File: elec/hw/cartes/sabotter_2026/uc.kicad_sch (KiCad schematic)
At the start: 34 parts, among them J3 USB4105-GF-A-060, SW1 TSB001A3526A02, U3 ESP32-S3-WROOM-1

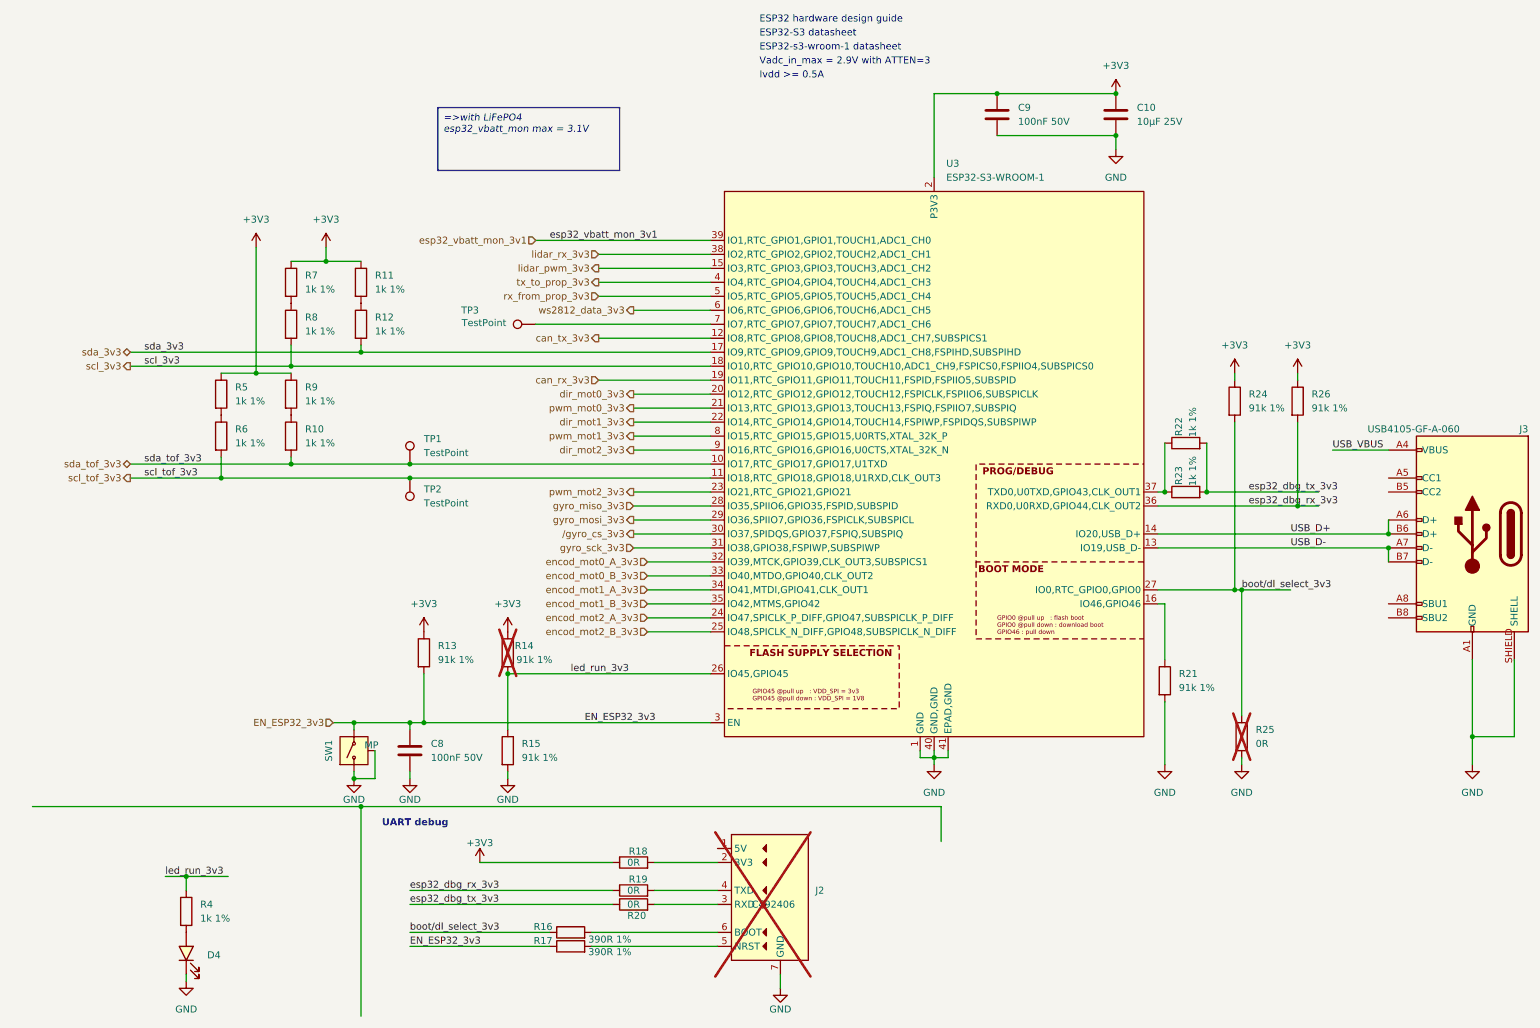
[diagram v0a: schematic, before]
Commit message: sabotter wip
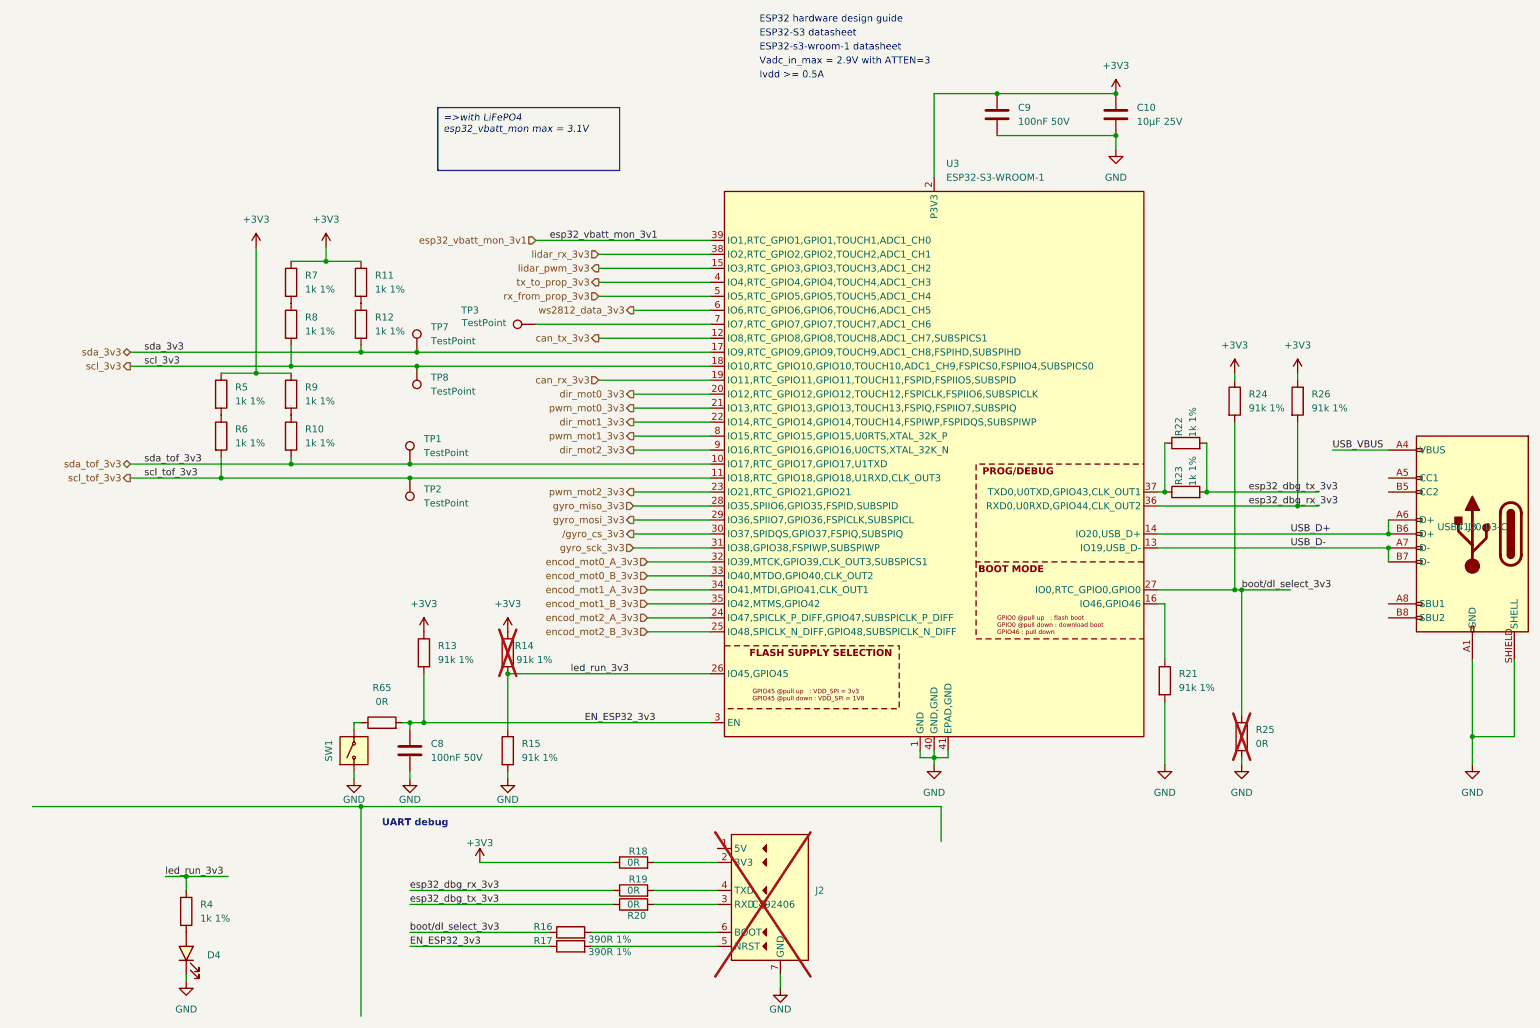
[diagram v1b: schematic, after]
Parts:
- added R65: 0R, cocotter_resistor:r0603_reflow, symbol cocotter_resistors:R_0R_0603
- added TP7, TP8: TestPoint, cocotter_others:testpoint-THT-0.5mm, symbol cocotter_others:TestPoint
- J3: value USB4105-GF-A-060 -> USB4120-03-C; footprint cocotter_connectors:USB4105 -> cocotter_connectors:USB4120-03-C; symbol cocotter_connectors:USB-TYPE-C-019 -> cocotter_connectors:USB4120-03-C; DIGIKEY_REF 2073-USB4105-GF-A-060TR-ND -> (none); JLC (none) -> C7450621; JLCPCB Part # C2927039 -> (none)
- SW1: value TSB001A3526A02 -> PTS525 SK15 SMTR2 LFS; footprint cocotter_others:TSB001A3526A02 -> cocotter_others:PTS525 SK15 SMTR2 LFS; symbol cocotter_others:TSB001A3526A02 -> cocotter_others:PTS525 SK15 SMTR2 LFS; JLCPCB Part # C2888889 -> C2689599
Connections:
- net EN_ESP32_3v3: now also R65.2; no longer SW1.2
- net GND: now also SW1.A (1); no longer SW1.1, SW1.MP
- net scl_3v3: now also TP8.1
- net sda_3v3: now also TP7.1
- new net: R65.1, SW1.B (2)

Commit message: sabotter wip
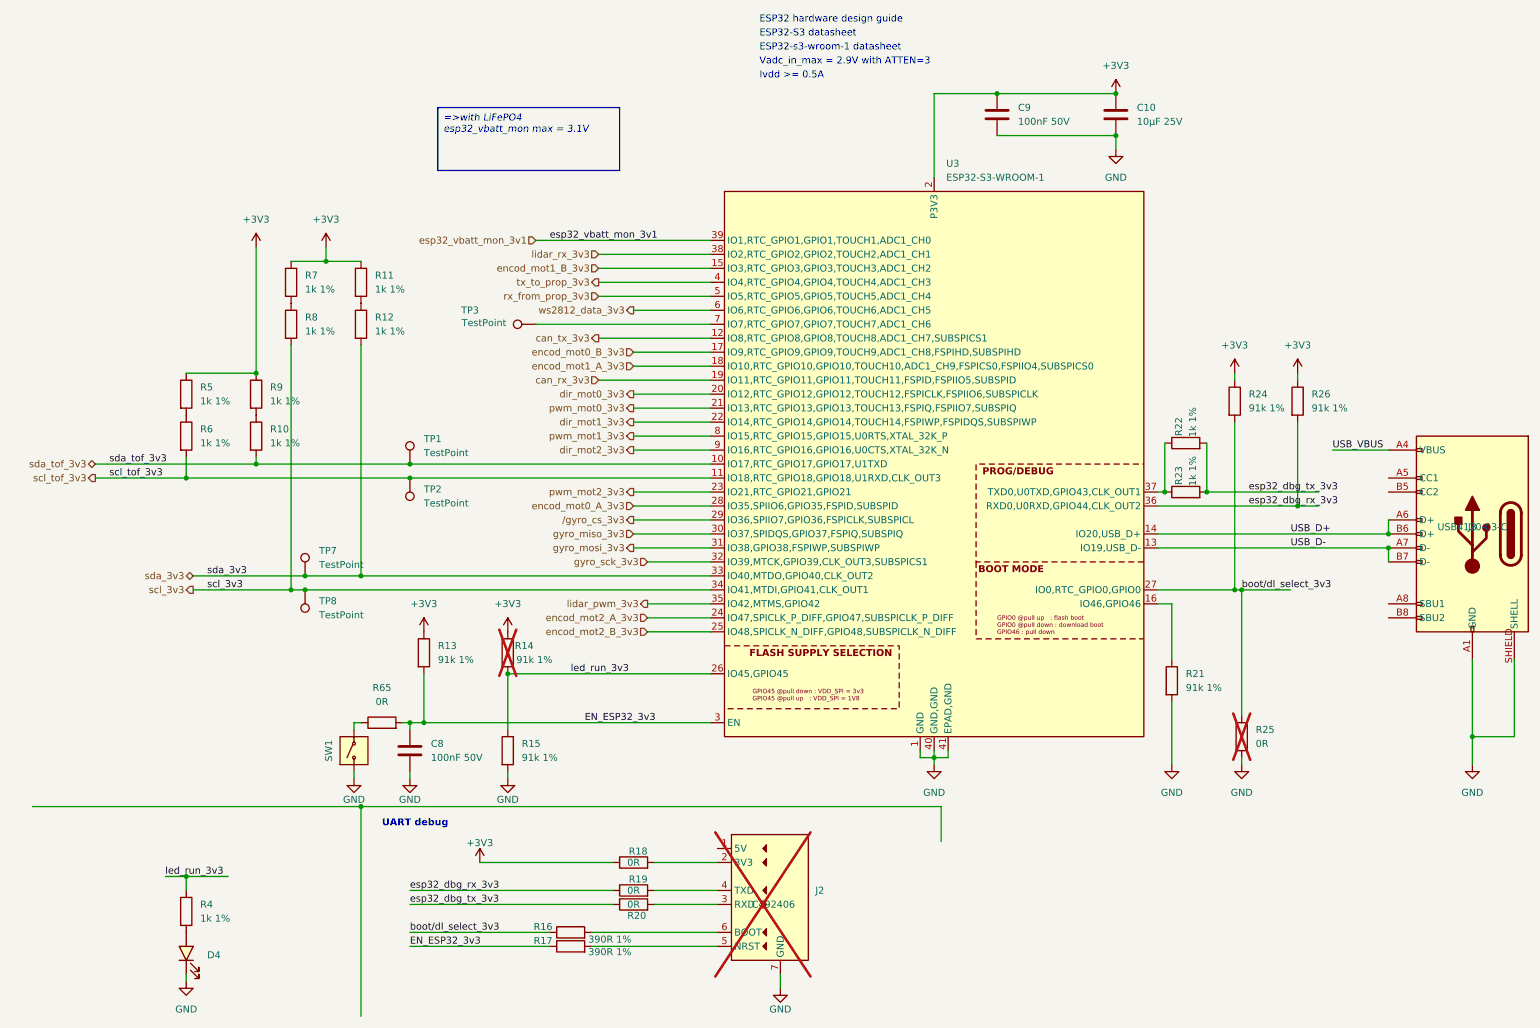
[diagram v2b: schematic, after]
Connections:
- net encod_mot0_A_3v3: now also U3.28 (IO35,SPIIO6,GPIO35,FSPID,SUBSPID); no longer U3.32 (IO39,MTCK,GPIO39,CLK_OUT3,SUBSPICS1)
- net encod_mot0_B_3v3: now also U3.17 (IO9,RTC_GPIO9,GPIO9,TOUCH9,ADC1_CH8,FSPIHD,SUBSPIHD); no longer U3.33 (IO40,MTDO,GPIO40,CLK_OUT2)
- net encod_mot1_A_3v3: now also U3.18 (IO10,RTC_GPIO10,GPIO10,TOUCH10,ADC1_CH9,FSPICS0,FSPIIO4,SUBSPICS0); no longer U3.34 (IO41,MTDI,GPIO41,CLK_OUT1)
- net encod_mot1_B_3v3: now also U3.15 (IO3,RTC_GPIO3,GPIO3,TOUCH3,ADC1_CH2); no longer U3.35 (IO42,MTMS,GPIO42)
- net gyro_miso_3v3: now also U3.30 (IO37,SPIDQS,GPIO37,FSPIQ,SUBSPIQ); no longer U3.28 (IO35,SPIIO6,GPIO35,FSPID,SUBSPID)
- net gyro_mosi_3v3: now also U3.31 (IO38,GPIO38,FSPIWP,SUBSPIWP); no longer U3.29 (IO36,SPIIO7,GPIO36,FSPICLK,SUBSPICL)
- net gyro_sck_3v3: now also U3.32 (IO39,MTCK,GPIO39,CLK_OUT3,SUBSPICS1); no longer U3.31 (IO38,GPIO38,FSPIWP,SUBSPIWP)
- net lidar_pwm_3v3: now also U3.35 (IO42,MTMS,GPIO42); no longer U3.15 (IO3,RTC_GPIO3,GPIO3,TOUCH3,ADC1_CH2)
- net scl_3v3: now also U3.34 (IO41,MTDI,GPIO41,CLK_OUT1); no longer U3.18 (IO10,RTC_GPIO10,GPIO10,TOUCH10,ADC1_CH9,FSPICS0,FSPIIO4,SUBSPICS0)
- net sda_3v3: now also U3.33 (IO40,MTDO,GPIO40,CLK_OUT2); no longer U3.17 (IO9,RTC_GPIO9,GPIO9,TOUCH9,ADC1_CH8,FSPIHD,SUBSPIHD)
- net /gyro_cs_3v3: now also U3.29 (IO36,SPIIO7,GPIO36,FSPICLK,SUBSPICL); no longer U3.30 (IO37,SPIDQS,GPIO37,FSPIQ,SUBSPIQ)
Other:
- moved on the sheet: R10, R21, R5, R6, R9, TP7, TP8

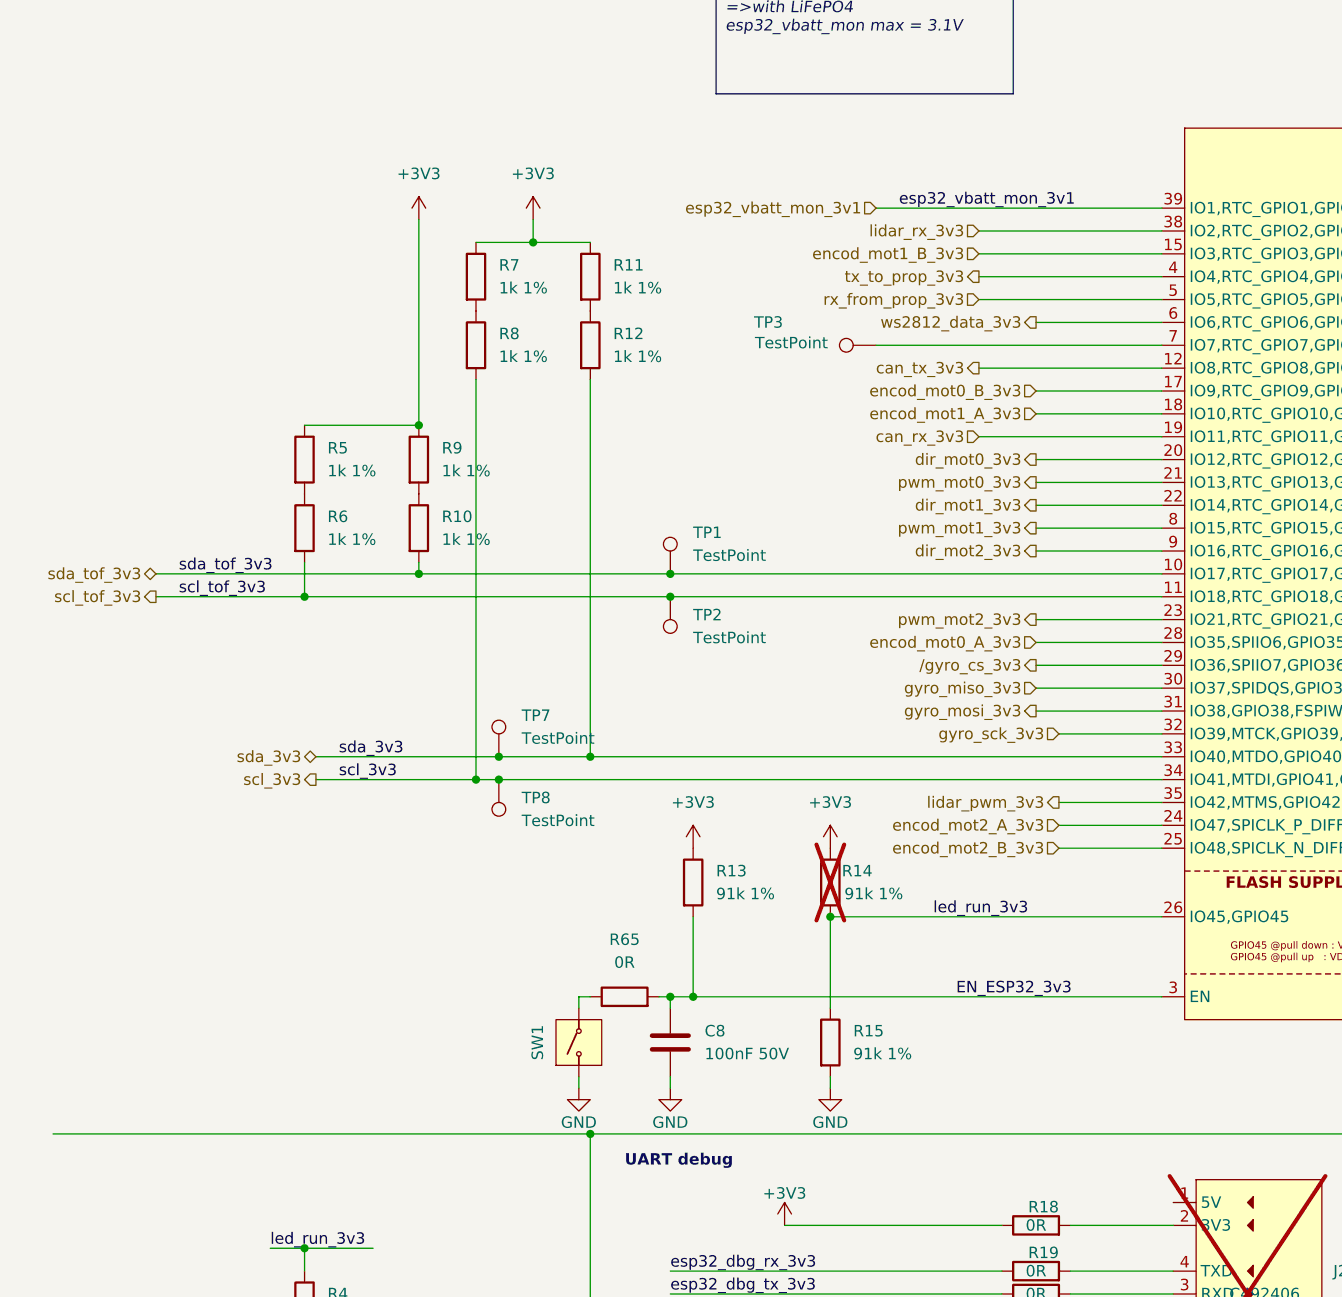
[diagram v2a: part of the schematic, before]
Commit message: sabotter ready for first schematic and routing review
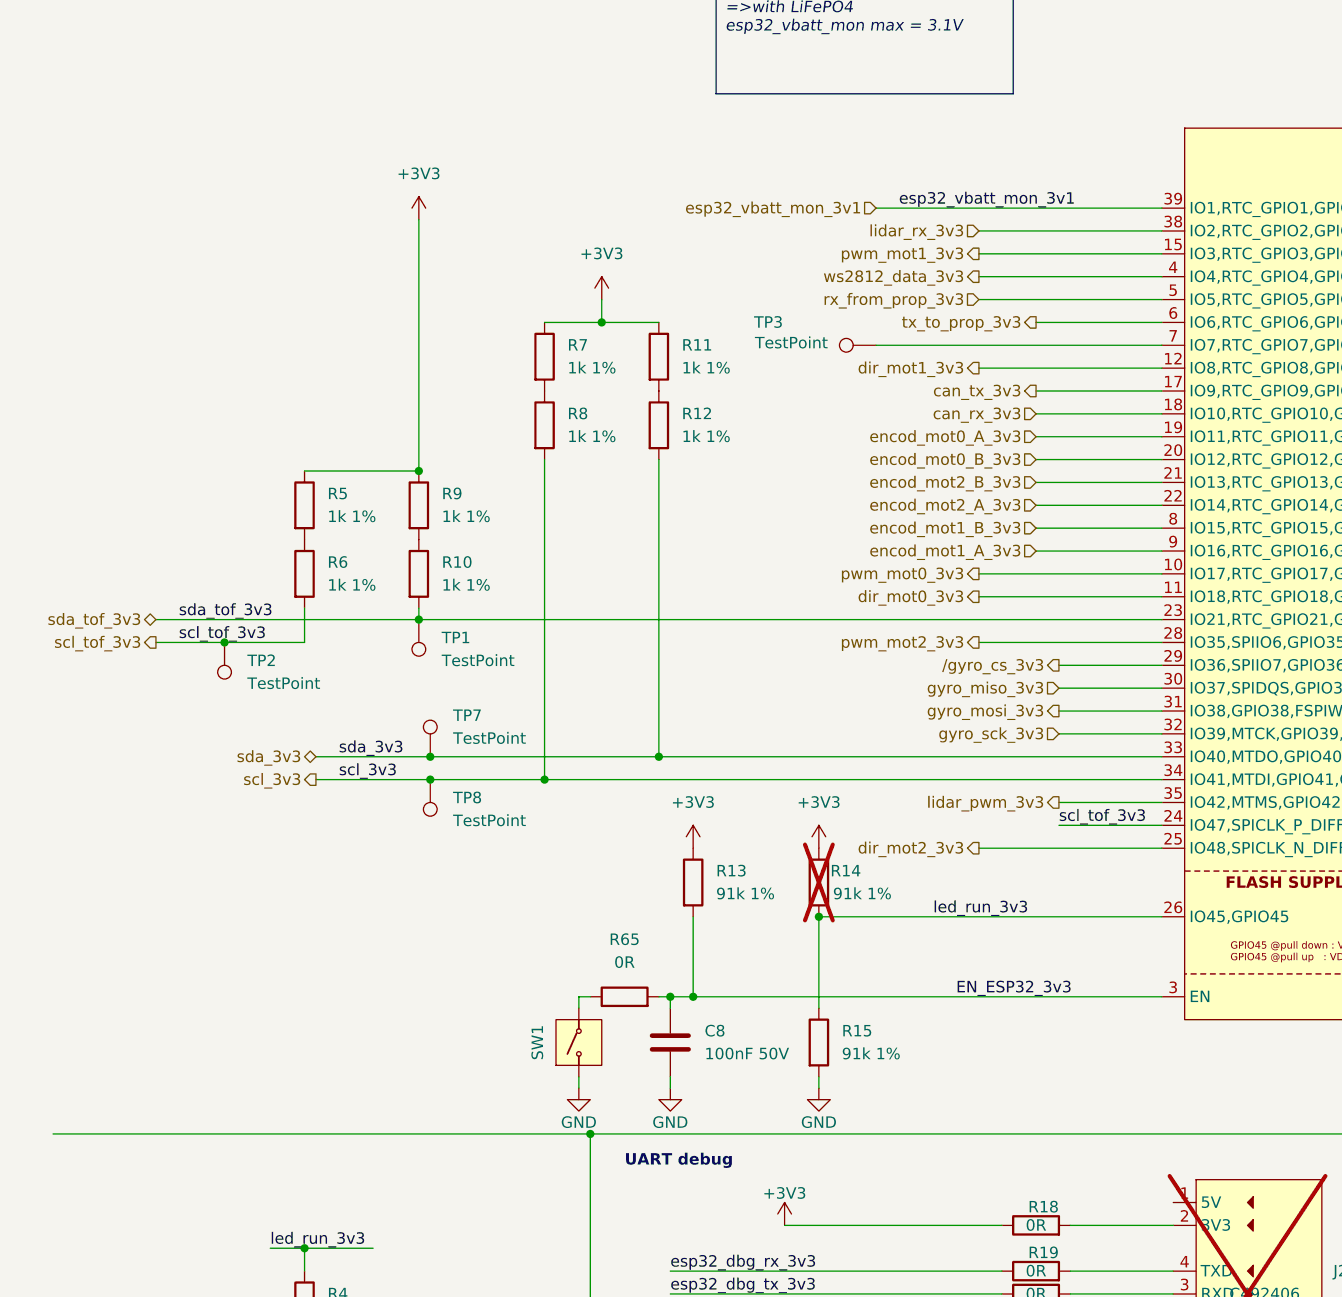
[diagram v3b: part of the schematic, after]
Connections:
- net can_rx_3v3: now also U3.18 (IO10,RTC_GPIO10,GPIO10,TOUCH10,ADC1_CH9,FSPICS0,FSPIIO4,SUBSPICS0); no longer U3.19 (IO11,RTC_GPIO11,GPIO11,TOUCH11,FSPID,FSPIIO5,SUBSPID)
- net can_tx_3v3: now also U3.17 (IO9,RTC_GPIO9,GPIO9,TOUCH9,ADC1_CH8,FSPIHD,SUBSPIHD); no longer U3.12 (IO8,RTC_GPIO8,GPIO8,TOUCH8,ADC1_CH7,SUBSPICS1)
- net dir_mot0_3v3: now also U3.11 (IO18,RTC_GPIO18,GPIO18,U1RXD,CLK_OUT3); no longer U3.20 (IO12,RTC_GPIO12,GPIO12,TOUCH12,FSPICLK,FSPIIO6,SUBSPICLK)
- net dir_mot1_3v3: now also U3.12 (IO8,RTC_GPIO8,GPIO8,TOUCH8,ADC1_CH7,SUBSPICS1); no longer U3.22 (IO14,RTC_GPIO14,GPIO14,TOUCH14,FSPIWP,FSPIDQS,SUBSPIWP)
- net dir_mot2_3v3: now also U3.25 (IO48,SPICLK_N_DIFF,GPIO48,SUBSPICLK_N_DIFF); no longer U3.9 (IO16,RTC_GPIO16,GPIO16,U0CTS,XTAL_32K_N)
- net encod_mot0_A_3v3: now also U3.19 (IO11,RTC_GPIO11,GPIO11,TOUCH11,FSPID,FSPIIO5,SUBSPID); no longer U3.28 (IO35,SPIIO6,GPIO35,FSPID,SUBSPID)
- net encod_mot0_B_3v3: now also U3.20 (IO12,RTC_GPIO12,GPIO12,TOUCH12,FSPICLK,FSPIIO6,SUBSPICLK); no longer U3.17 (IO9,RTC_GPIO9,GPIO9,TOUCH9,ADC1_CH8,FSPIHD,SUBSPIHD)
- net encod_mot1_A_3v3: now also U3.9 (IO16,RTC_GPIO16,GPIO16,U0CTS,XTAL_32K_N); no longer U3.18 (IO10,RTC_GPIO10,GPIO10,TOUCH10,ADC1_CH9,FSPICS0,FSPIIO4,SUBSPICS0)
- net encod_mot1_B_3v3: now also U3.8 (IO15,RTC_GPIO15,GPIO15,U0RTS,XTAL_32K_P); no longer U3.15 (IO3,RTC_GPIO3,GPIO3,TOUCH3,ADC1_CH2)
- net encod_mot2_A_3v3: now also U3.22 (IO14,RTC_GPIO14,GPIO14,TOUCH14,FSPIWP,FSPIDQS,SUBSPIWP); no longer U3.24 (IO47,SPICLK_P_DIFF,GPIO47,SUBSPICLK_P_DIFF)
- net encod_mot2_B_3v3: now also U3.21 (IO13,RTC_GPIO13,GPIO13,TOUCH13,FSPIQ,FSPIIO7,SUBSPIQ); no longer U3.25 (IO48,SPICLK_N_DIFF,GPIO48,SUBSPICLK_N_DIFF)
- net pwm_mot0_3v3: now also U3.10 (IO17,RTC_GPIO17,GPIO17,U1TXD); no longer U3.21 (IO13,RTC_GPIO13,GPIO13,TOUCH13,FSPIQ,FSPIIO7,SUBSPIQ)
- net pwm_mot1_3v3: now also U3.15 (IO3,RTC_GPIO3,GPIO3,TOUCH3,ADC1_CH2); no longer U3.8 (IO15,RTC_GPIO15,GPIO15,U0RTS,XTAL_32K_P)
- net pwm_mot2_3v3: now also U3.28 (IO35,SPIIO6,GPIO35,FSPID,SUBSPID); no longer U3.23 (IO21,RTC_GPIO21,GPIO21)
- net scl_tof_3v3: now also U3.24 (IO47,SPICLK_P_DIFF,GPIO47,SUBSPICLK_P_DIFF); no longer U3.11 (IO18,RTC_GPIO18,GPIO18,U1RXD,CLK_OUT3)
- net sda_tof_3v3: now also U3.23 (IO21,RTC_GPIO21,GPIO21); no longer U3.10 (IO17,RTC_GPIO17,GPIO17,U1TXD)
- net tx_to_prop_3v3: now also U3.6 (IO6,RTC_GPIO6,GPIO6,TOUCH6,ADC1_CH5); no longer U3.4 (IO4,RTC_GPIO4,GPIO4,TOUCH4,ADC1_CH3)
- net ws2812_data_3v3: now also U3.4 (IO4,RTC_GPIO4,GPIO4,TOUCH4,ADC1_CH3); no longer U3.6 (IO6,RTC_GPIO6,GPIO6,TOUCH6,ADC1_CH5)
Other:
- moved on the sheet: R10, R11, R12, R14, R15, R5, R6, R7, R8, R9, TP1, TP2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
